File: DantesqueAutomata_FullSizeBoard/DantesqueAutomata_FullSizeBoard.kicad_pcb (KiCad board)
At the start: 2 copper layers, 90 x 110 mm, 112 parts, among them J1 DantesqueAutomata-Connector, J2 EurorackPower-Connector, U1 ESP32-DevKitC, U10 LM833, U11 LM833, U12 LM833, U2 GY-PCM5102, U3 GY-PCM5102, U4 LM833, U5 LM833, U6 LM833, U7 CJMCU-1808, U8 CJMCU-1808, U9 LM833

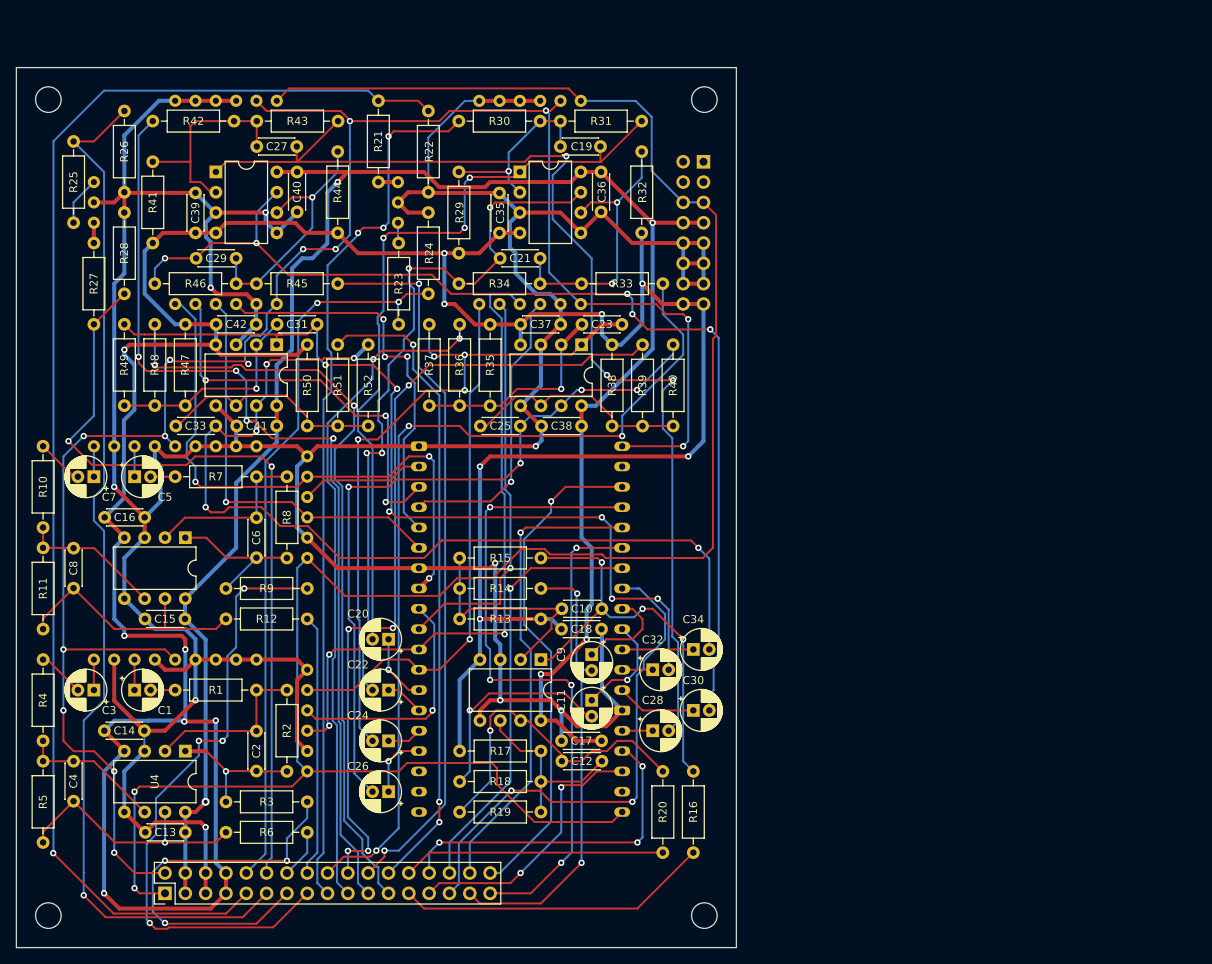
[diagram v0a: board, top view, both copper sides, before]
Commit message: improved pcb design of full size board
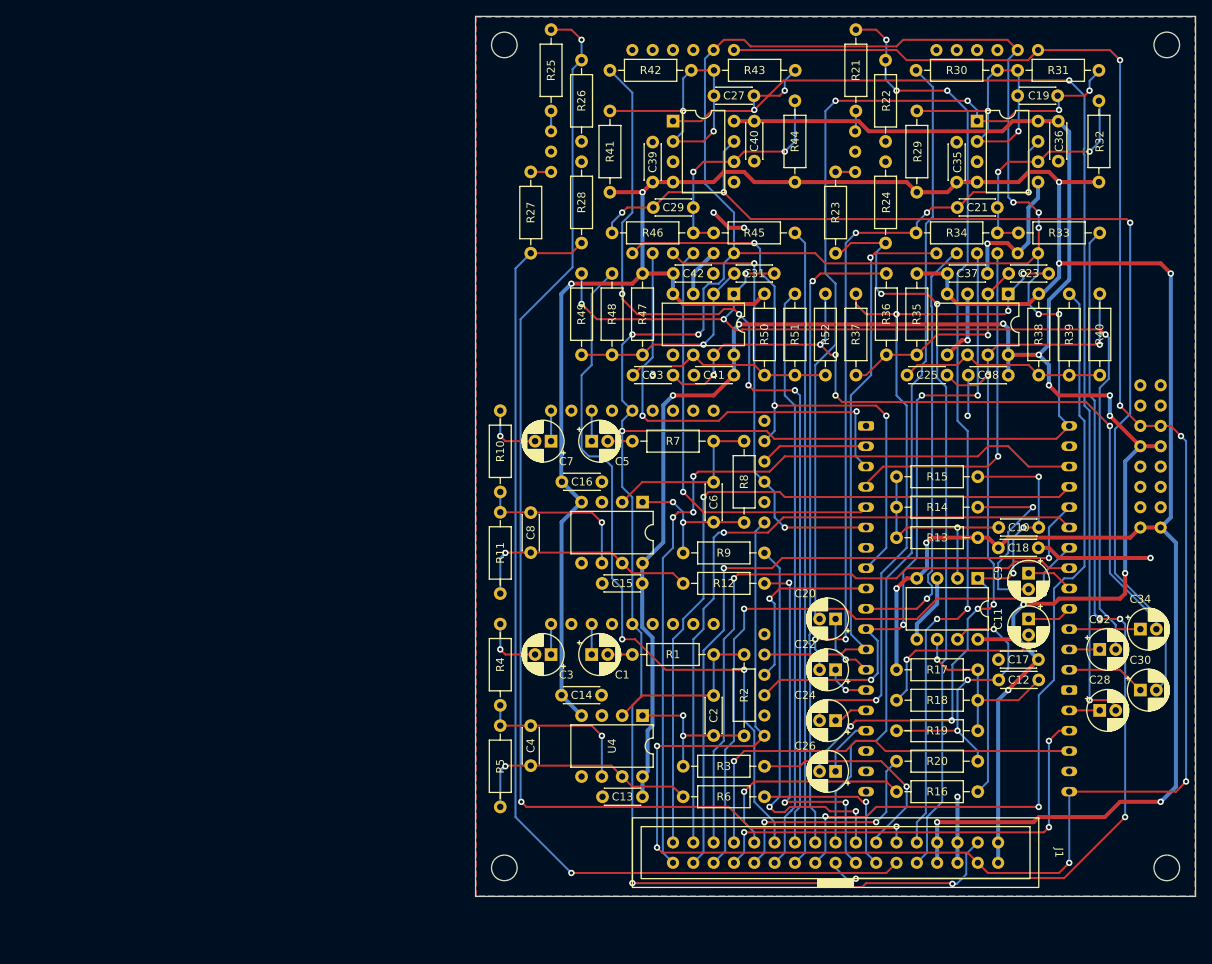
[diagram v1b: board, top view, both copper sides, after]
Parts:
- removed the REF** at (136.0, 159.0)
- removed the REF** at (136.0, 57.0)
- removed the REF** at (54.0, 159.0)
- removed the REF** at (54.0, 57.0)
- added REF**: MountingHole_3.2mm_M3, MountingHole:MountingHole_3.2mm_M3, F.Cu at (111.0, 50.2)
- added REF**: MountingHole_3.2mm_M3, MountingHole:MountingHole_3.2mm_M3, F.Cu at (111.0, 153.0)
- added REF**: MountingHole_3.2mm_M3, MountingHole:MountingHole_3.2mm_M3, F.Cu at (193.8, 50.2)
- added REF**: MountingHole_3.2mm_M3, MountingHole:MountingHole_3.2mm_M3, F.Cu at (193.8, 153.0)
- J1: value DantesqueAutomata-Connector -> Dantesque_Automata_Connector; footprint Connector_PinHeader_2.54mm:PinHeader_2x17_P2.54mm_Vertical -> Connector_Eurorack:Dantesque_Automata_Connector
- J2: value EurorackPower-Connector -> Eurorack_16_Pin_Power; footprint Connector_PinHeader_2.54mm:PinHeader_2x08_P2.54mm_Vertical -> Connector_Eurorack:Eurorack_16_Pin_Power
- moved J1 84.0 mm to (152.4, 151.1), turned to -90 degrees
- moved J2 66.9 mm to (191.8, 101.6)
- moved R25 61.3 mm to (116.8, 48.3)
- moved R21 60.3 mm to (154.9, 48.3)
- moved R29 57.8 mm to (162.6, 68.6)
- moved U7 57.5 mm to (171.4, 63.5)
- moved C21 57.5 mm to (172.6, 70.5)
- moved C29 57.5 mm to (134.6, 70.5)
- moved C31 57.5 mm to (139.7, 78.7)
- moved C36 57.5 mm to (180.2, 64.7)
- moved C40 57.5 mm to (142.2, 64.7)
- moved C42 57.5 mm to (132.1, 78.7)
- moved R22 57.5 mm to (158.7, 62.2)
- moved R24 57.5 mm to (158.7, 64.8)
- moved R26 57.5 mm to (120.7, 62.2)
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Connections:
- net ADC_1 renamed ADC1
- net ADC_2 renamed ADC2
- net ADC_3 renamed ADC3
- net ADC_4 renamed ADC4
- net ADC_5 renamed ADC5
- net ADC_6 renamed ADC6
- net ADC_7 renamed ADC7
- net ADC_8 renamed ADC8
- net BCK_1 renamed BCK1
- net BCK_2 renamed BCK2
- net DAC_1 renamed DAC1
- net DAC_2 renamed DAC2
- net DIN_1 renamed DIN1
- net DIN_2 renamed DIN2
- net DOUT_1 renamed DOUT1
- net DOUT_2 renamed DOUT2
- net GPIO_1 renamed GPIO1
- net GPIO_2 renamed GPIO2
- net GPIO_3 renamed GPIO3
- net GPIO_4 renamed GPIO4
- net GPIO_5 renamed GPIO5
- net GPIO_6 renamed GPIO6
- net GPIO_7 renamed GPIO7
- net GPIO_8 renamed GPIO8
- net LD_A_IN_1 renamed LD_A_IN1
- net LD_A_IN_2 renamed LD_A_IN2
- net LD_A_IN_3 renamed LD_A_IN3
- net LD_A_IN_4 renamed LD_A_IN4
- net LD_A_IN_5 renamed LD_A_IN5
- net LD_A_IN_6 renamed LD_A_IN6
- net LD_A_IN_7 renamed LD_A_IN7
- net LD_A_IN_8 renamed LD_A_IN8
- net LD_A_OUT_1 renamed LD_A_OUT1
- net LD_A_OUT_2 renamed LD_A_OUT2
- net LIN_1 renamed LIN1
- net LIN_2 renamed LIN2
- net L_OUT_1 renamed LOUT1
- net L_OUT_2 renamed LOUT2
- net MCK_1 renamed MCK1
- net MCK_2 renamed MCK2
- net RIN_1 renamed RIN1
- net RIN_2 renamed RIN2
- net R_OUT_1 renamed ROUT1
- net R_OUT_2 renamed ROUT2
- net WS_1 renamed WS1
- net WS_2 renamed WS2
- J1 pad 1: +5V -> +12V
- J1 pad 2: +3.3V -> +12V
- J1 pad 3: +12V -> +3.3V
- J1 pad 4: +12V -> +5V
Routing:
- net GND: track 509.2 -> 74.6 mm, vias 9 -> 8
- net +3.3V: track 254.0 -> 357.3 mm, vias 14 -> 10
- net HD_A_IN1: track 167.8 -> 117.8 mm, vias 1 -> 5
- net +12V: track 239.3 -> 281.3 mm, vias 5 -> 11
- net GPIO8: track 62.7 -> 101.2 mm, vias 1 -> 3
- net HD_A_OUT3: track 78.5 -> 48.5 mm, vias 4 -> 2
- net HD_A_IN4: track 100.0 -> 129.2 mm, vias 2 -> 1
- net GPIO6: track 59.2 -> 87.0 mm, vias 1 -> 2
- net GPIO4: track 53.7 -> 79.7 mm, vias 1 -> 2
- net GPIO5: track 62.5 -> 85.2 mm, vias 2 -> 1
- net HD_A_IN3: track 131.1 -> 153.1 mm, vias 1 -> 3
- net HD_A_OUT1: track 49.7 -> 27.9 mm, vias 3 -> 1
- net GPIO1: track 33.7 -> 53.6 mm, vias 2 -> 1
- net -12V: track 380.4 -> 361.6 mm, vias 13 -> 9
- net Net-(C33-Pad2): track 118.4 -> 100.2 mm
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- added copper zone on B.Cu, net GND
- added copper zone on F.Cu, net GND
